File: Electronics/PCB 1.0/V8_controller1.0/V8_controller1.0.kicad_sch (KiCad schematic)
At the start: 14 parts, among them Q1 IRLZ34N, SW1 SW_SPST, U1 LM317_TO-263, U2 LM317_TO-263

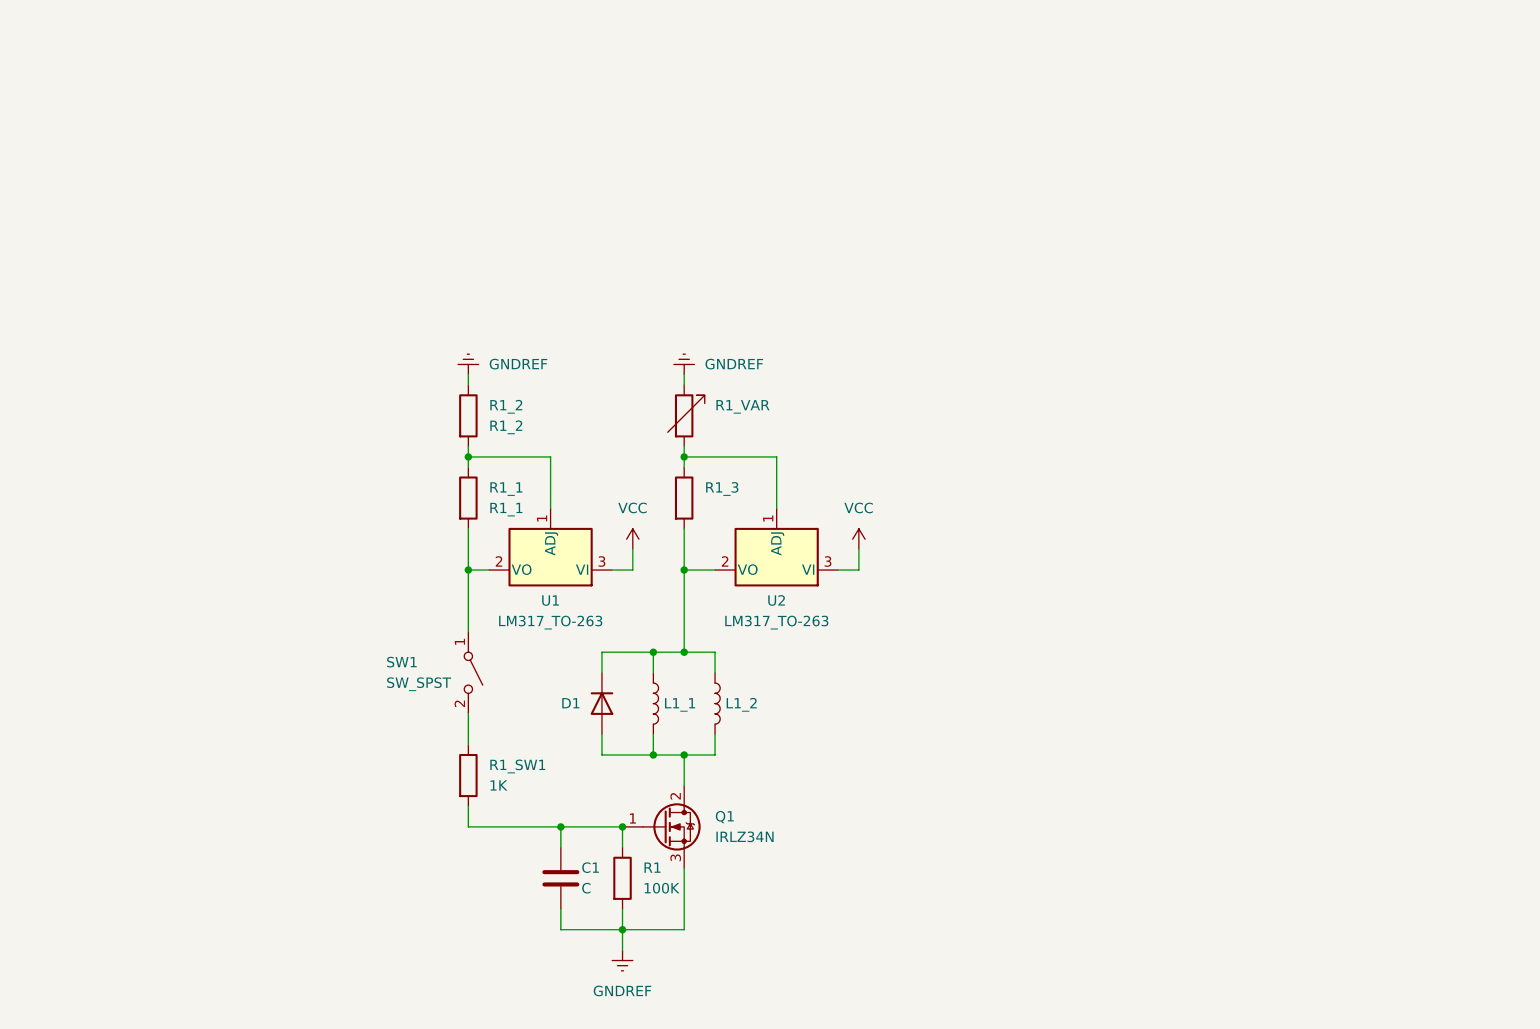
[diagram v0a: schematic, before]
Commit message: Add final gerberfiles for 1.0
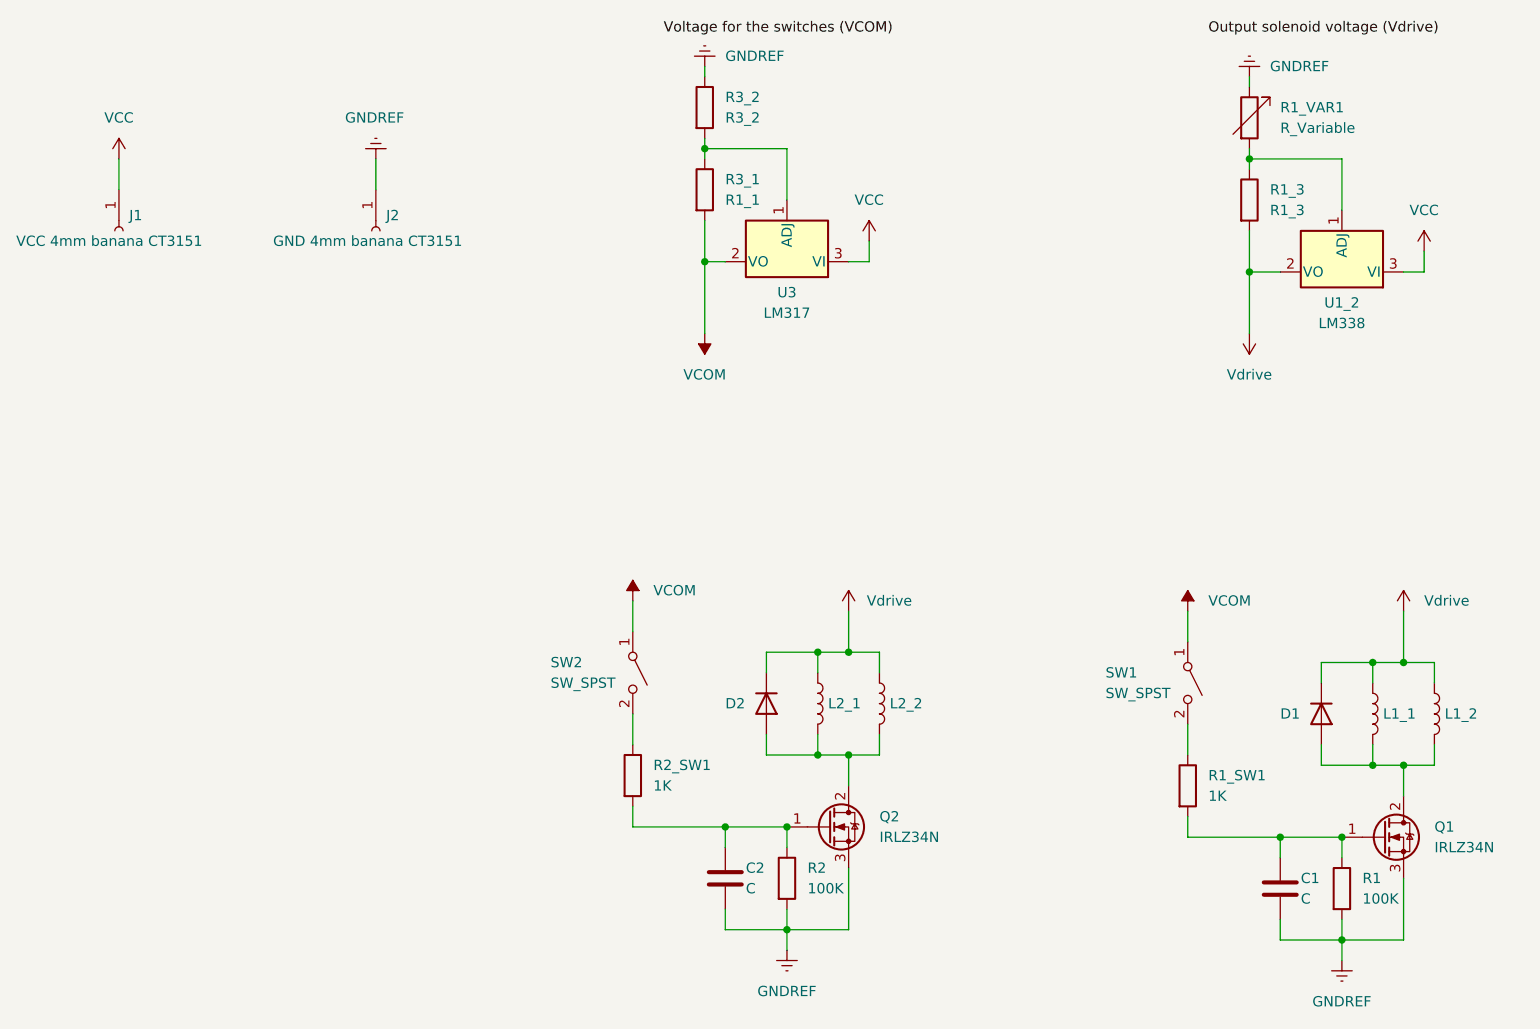
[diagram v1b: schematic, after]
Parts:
- removed R1_1: R1_1, Resistor_SMD:R_0805_2012Metric_Pad1.20x1.40mm_HandSolder, symbol Device:R
- removed R1_2: R1_2, Resistor_SMD:R_0805_2012Metric_Pad1.20x1.40mm_HandSolder, symbol Device:R
- removed U1: LM317_TO-263, Package_TO_SOT_SMD:TO-263-2, symbol Regulator_Linear:LM317_TO-263
- added C2: C, Resistor_SMD:R_0805_2012Metric_Pad1.20x1.40mm_HandSolder, symbol Device:C
- added D2: DIODE, Diode_SMD:D_SMA-SMB_Universal_Handsoldering, symbol Simulation_SPICE:DIODE
- added J1: VCC 4mm banana CT3151, Connector:CalTest_CT3151, symbol Connector:Conn_01x01_Female
- added J2: GND 4mm banana CT3151, Connector:CalTest_CT3151, symbol Connector:Conn_01x01_Female
- added L2_1, L2_2: L, Connector_JST:JST_EH_S2B-EH_1x02_P2.50mm_Horizontal, symbol Device:L
- added Q2: IRLZ34N, Package_TO_SOT_THT:TO-220-3_Horizontal_TabDown, symbol Transistor_FET:IRLZ34N
- added R2: 100K, Resistor_SMD:R_0805_2012Metric_Pad1.20x1.40mm_HandSolder, symbol Device:R
- added R2_SW1: 1K, Resistor_SMD:R_0805_2012Metric_Pad1.20x1.40mm_HandSolder, symbol Device:R
- added R3_1: R1_1, Resistor_SMD:R_0805_2012Metric_Pad1.20x1.40mm_HandSolder, symbol Device:R
- added R3_2: R3_2, Resistor_SMD:R_0805_2012Metric_Pad1.20x1.40mm_HandSolder, symbol Device:R
- added SW2: SW_SPST, Connector_JST:JST_EH_S2B-EH_1x02_P2.50mm_Horizontal, symbol Switch:SW_SPST
- added U3: LM317, Package_TO_SOT_SMD:TO-263-2, symbol Regulator_Linear:LM317_TO-263
- R1_3: value (none) -> R1_3
- R1_VAR1: renamed from R1_VAR; value (none) -> R_Variable; footprint (none) -> Resistor_THT:R_Axial_DIN0204_L3.6mm_D1.6mm_P1.90mm_Vertical
- U1_2: renamed from U2; value LM317_TO-263 -> LM338; footprint Package_TO_SOT_SMD:TO-263-2 -> Package_TO_SOT_THT:TO-220-3_Horizontal_TabDown
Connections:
- net GNDREF: now also C2.2, J2.1 (Pin_1), Q2.3 (S), R2.2, R3_2.1
- net VCC: now also J1.1 (Pin_1), U3.3 (VI)
- net Vdrive: now reaches D1.2 (K), L1_1.1, L1_2.1, R1_3.2, U1_2.2 (VO)
- net Vdrive: now also D2.2 (K), L2_1.1, L2_2.1
- net VCOM: now reaches SW1.1 (A)
- net VCOM: now also R3_1.2, SW2.1 (A), U3.2 (VO)
- new net: C2.1, Q2.1 (G), R2.1, R2_SW1.2
- new net: D2.1 (A), L2_1.2, L2_2.2, Q2.2 (D)
- new net: R2_SW1.1, SW2.2 (B)
- new net: R3_1.1, R3_2.2, U3.1 (ADJ)
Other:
- moved on the sheet: C1, D1, L1_1, L1_2, Q1, R1, R1_3, R1_SW1, R1_VAR1, SW1, U1_2
